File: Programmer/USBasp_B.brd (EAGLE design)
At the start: 25.7 x 64.6 mm, 20 parts, among them IC1 ATMega8, Q1 12MHz

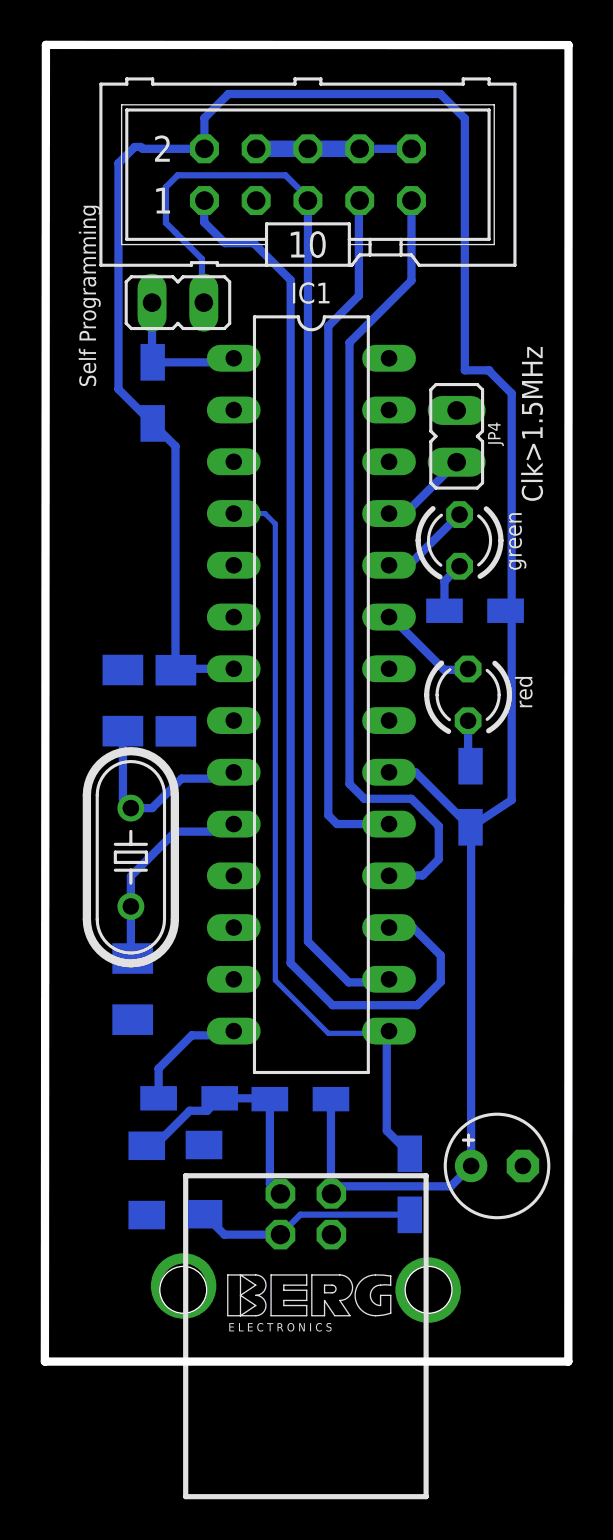
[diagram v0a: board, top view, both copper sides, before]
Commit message: Add files via upload
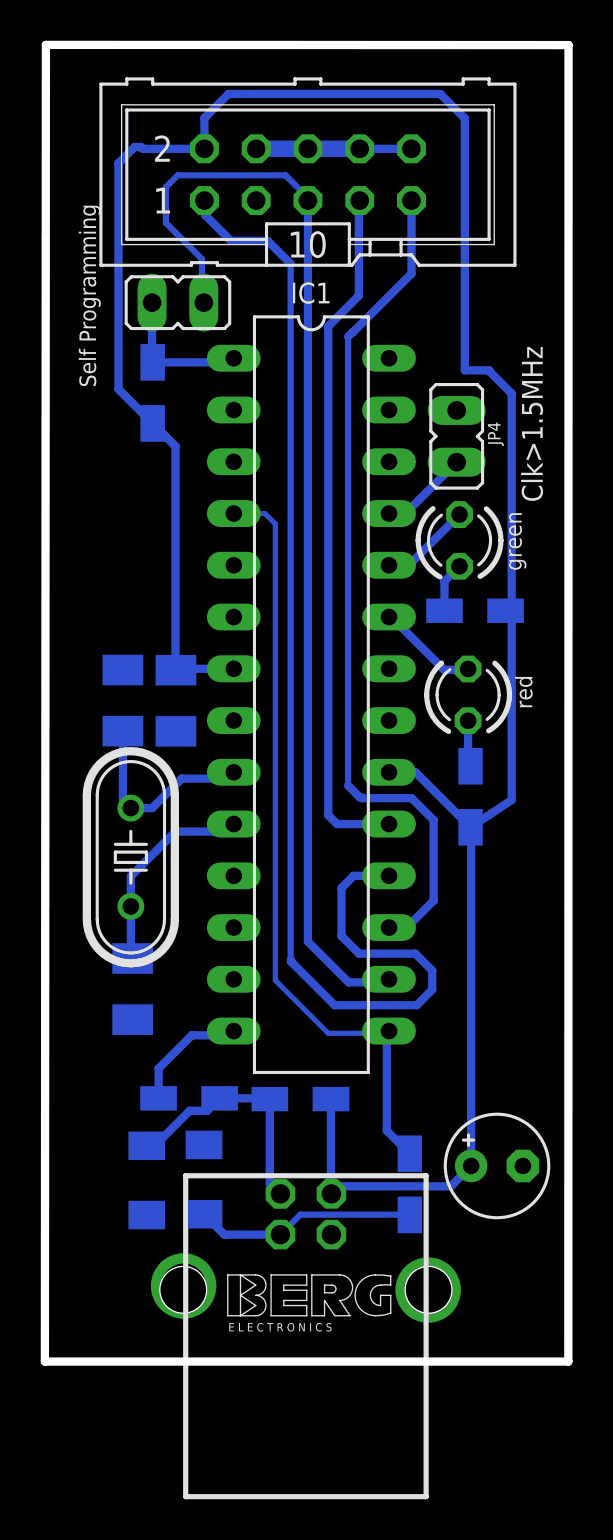
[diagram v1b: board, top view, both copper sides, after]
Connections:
- net N$27: now also X2.1; no longer X2.9
- net N$3: now also X2.9; no longer X2.1
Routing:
- net N$27: track 39.5 -> 59.3 mm
- net N$3: track 53.1 -> 41.6 mm
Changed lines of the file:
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@@
 </polygon>
 <contactref element="JP4" pad="2"/>
-<wire x1="9.66" y1="31.55" x2="17.28" y2="34.09" width="0" layer="19" extent="1-1"/>
+<wire x1="17.28" y1="34.09" x2="9.66" y2="31.55" width="0" layer="19" extent="1-1"/>
 </signal>
 <signal name="N$5">
@@
 <wire x1="8.969" y1="13.01" x2="11.391" y2="13.01" width="0.4064" layer="16"/>
 <wire x1="11.391" y1="13.01" x2="11.431" y2="12.97" width="0.4064" layer="16"/>
-<wire x1="5.39" y1="10.68" x2="5.78" y2="10.68" width="0.4064" layer="16"/>
 <wire x1="5.78" y1="10.68" x2="7.5" y2="12.4" width="0.4064" layer="16"/>
 <wire x1="7.5" y1="12.4" x2="8.359" y2="12.4" width="0.4064" layer="16"/>
 <wire x1="8.359" y1="12.4" x2="8.969" y2="13.01" width="0.4064" layer="16"/>
+<wire x1="5.39" y1="10.68" x2="5.78" y2="10.68" width="0.4064" layer="16"/>
 </signal>
 <signal name="N$8">
@@
 <wire x1="9.45" y1="16.1" x2="9.66" y2="16.31" width="0.4064" layer="16"/>
 </signal>
-<signal name="N$3">
-<contactref element="X2" pad="1"/>
-<contactref element="IC1" pad="17"/>
-<wire x1="17.28" y1="21.39" x2="18.45" y2="21.39" width="0.4064" layer="16"/>
-<wire x1="18.45" y1="21.39" x2="19.82" y2="20.02" width="0.4064" layer="16"/>
-<wire x1="19.82" y1="20.02" x2="19.82" y2="18.72" width="0.4064" layer="16"/>
-<wire x1="19.82" y1="18.72" x2="18.75" y2="17.65" width="0.4064" layer="16"/>
-<wire x1="18.75" y1="17.65" x2="18.74" y2="17.65" width="0.4064" layer="16"/>
-<wire x1="18.74" y1="17.65" x2="18.67" y2="17.58" width="0.4064" layer="16"/>
-<wire x1="18.67" y1="17.58" x2="14.51" y2="17.58" width="0.4064" layer="16"/>
-<wire x1="14.51" y1="17.58" x2="12.45" y2="19.64" width="0.4064" layer="16"/>
-<wire x1="12.45" y1="19.64" x2="12.45" y2="53.17" width="0.4064" layer="16"/>
-<wire x1="12.45" y1="53.17" x2="10.64" y2="54.98" width="0.4064" layer="16"/>
-<wire x1="10.64" y1="54.98" x2="9.23" y2="54.98" width="0.4064" layer="16"/>
-<wire x1="9.23" y1="54.98" x2="8.21" y2="56" width="0.4064" layer="16"/>
-<wire x1="8.21" y1="56" x2="8.21" y2="57.06" width="0.4064" layer="16"/>
-<wire x1="8.21" y1="57.06" x2="8.22" y2="57.07" width="0.4064" layer="16"/>
-</signal>
 <signal name="N$9">
 </signal>
@@
 <signal name="N$27">
 <contactref element="IC1" pad="18"/>
+<contactref element="X2" pad="1"/>
+<wire x1="17.28" y1="23.93" x2="15.55" y2="23.93" width="0.4064" layer="16"/>
+<wire x1="15.55" y1="23.93" x2="14.95" y2="23.33" width="0.4064" layer="16"/>
+<wire x1="14.95" y1="23.33" x2="14.95" y2="20.97" width="0.4064" layer="16"/>
+<wire x1="14.95" y1="20.97" x2="15.81" y2="20.11" width="0.4064" layer="16"/>
+<wire x1="15.81" y1="20.11" x2="18.57" y2="20.11" width="0.4064" layer="16"/>
+<wire x1="18.57" y1="20.11" x2="19.4" y2="19.28" width="0.4064" layer="16"/>
+<wire x1="19.4" y1="19.28" x2="19.4" y2="18.34" width="0.4064" layer="16"/>
+<wire x1="19.4" y1="18.34" x2="18.64" y2="17.58" width="0.4064" layer="16"/>
+<wire x1="18.64" y1="17.58" x2="14.61" y2="17.58" width="0.4064" layer="16"/>
+<wire x1="14.61" y1="17.58" x2="12.48" y2="19.71" width="0.4064" layer="16"/>
+<wire x1="12.48" y1="19.71" x2="12.48" y2="19.76" width="0.4064" layer="16"/>
+<wire x1="12.48" y1="19.76" x2="12.45" y2="19.79" width="0.4064" layer="16"/>
+<wire x1="12.45" y1="19.79" x2="12.45" y2="53.97" width="0.3048" layer="16"/>
+<wire x1="12.45" y1="53.97" x2="11.33" y2="55.09" width="0.4064" layer="16"/>
+<wire x1="11.33" y1="55.09" x2="9.52" y2="55.09" width="0.4064" layer="16"/>
+<wire x1="9.52" y1="55.09" x2="8.25" y2="56.36" width="0.4064" layer="16"/>
+<wire x1="8.25" y1="56.36" x2="8.25" y2="57.04" width="0.4064" layer="16"/>
+<wire x1="8.25" y1="57.04" x2="8.22" y2="57.07" width="0.4064" layer="16"/>
+</signal>
+<signal name="N$3">
 <contactref element="X2" pad="9"/>
-<wire x1="18.38" y1="57.07" x2="18.38" y2="53.14" width="0.4064" layer="16"/>
-<wire x1="18.38" y1="53.14" x2="15.34" y2="50.1" width="0.4064" layer="16"/>
-<wire x1="15.34" y1="50.1" x2="15.34" y2="28.44" width="0.4064" layer="16"/>
-<wire x1="15.34" y1="28.44" x2="16.07" y2="27.71" width="0.4064" layer="16"/>
-<wire x1="16.07" y1="27.71" x2="18.38" y2="27.71" width="0.4064" layer="16"/>
-<wire x1="18.38" y1="27.71" x2="19.72" y2="26.37" width="0.4064" layer="16"/>
-<wire x1="19.72" y1="26.37" x2="19.72" y2="24.74" width="0.4064" layer="16"/>
-<wire x1="19.72" y1="24.74" x2="18.93" y2="23.95" width="0.4064" layer="16"/>
-<wire x1="18.93" y1="23.95" x2="17.3" y2="23.95" width="0.4064" layer="16"/>
-<wire x1="17.3" y1="23.95" x2="17.28" y2="23.93" width="0.4064" layer="16"/>
+<contactref element="IC1" pad="17"/>
+<wire x1="18.38" y1="57.07" x2="18.38" y2="53.48" width="0.4064" layer="16"/>
+<wire x1="18.38" y1="53.48" x2="15.51" y2="50.61" width="0.4064" layer="16"/>
+<wire x1="15.51" y1="50.61" x2="15.49" y2="50.61" width="0.4064" layer="16"/>
+<wire x1="15.49" y1="50.61" x2="15.27" y2="50.39" width="0.4064" layer="16"/>
+<wire x1="15.27" y1="50.39" x2="15.27" y2="28.36" width="0.3048" layer="16"/>
+<wire x1="15.27" y1="28.36" x2="15.85" y2="27.78" width="0.4064" layer="16"/>
+<wire x1="15.85" y1="27.78" x2="15.88" y2="27.78" width="0.4064" layer="16"/>
+<wire x1="15.88" y1="27.78" x2="15.92" y2="27.74" width="0.4064" layer="16"/>
+<wire x1="15.92" y1="27.74" x2="18.39" y2="27.74" width="0.4064" layer="16"/>
+<wire x1="18.39" y1="27.74" x2="19.47" y2="26.66" width="0.4064" layer="16"/>
+<wire x1="19.47" y1="26.66" x2="19.47" y2="22.71" width="0.4064" layer="16"/>
+<wire x1="19.47" y1="22.71" x2="18.17" y2="21.41" width="0.4064" layer="16"/>
+<wire x1="18.17" y1="21.41" x2="17.3" y2="21.41" width="0.4064" layer="16"/>
+<wire x1="17.3" y1="21.41" x2="17.28" y2="21.39" width="0.4064" layer="16"/>
 </signal>
 </signals>
